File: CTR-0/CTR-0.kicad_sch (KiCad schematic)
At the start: 34 parts, among them J1 USB_C_Receptacle_USB2.0_14P, J2 Conn_01x20, J3 Conn_01x20, J4 Conn_01x03, SW1 SW_Push, U1 RP2040, U2 NCP1117-3.3_SOT223, U3 W25Q128JVS, Y1 12MHz

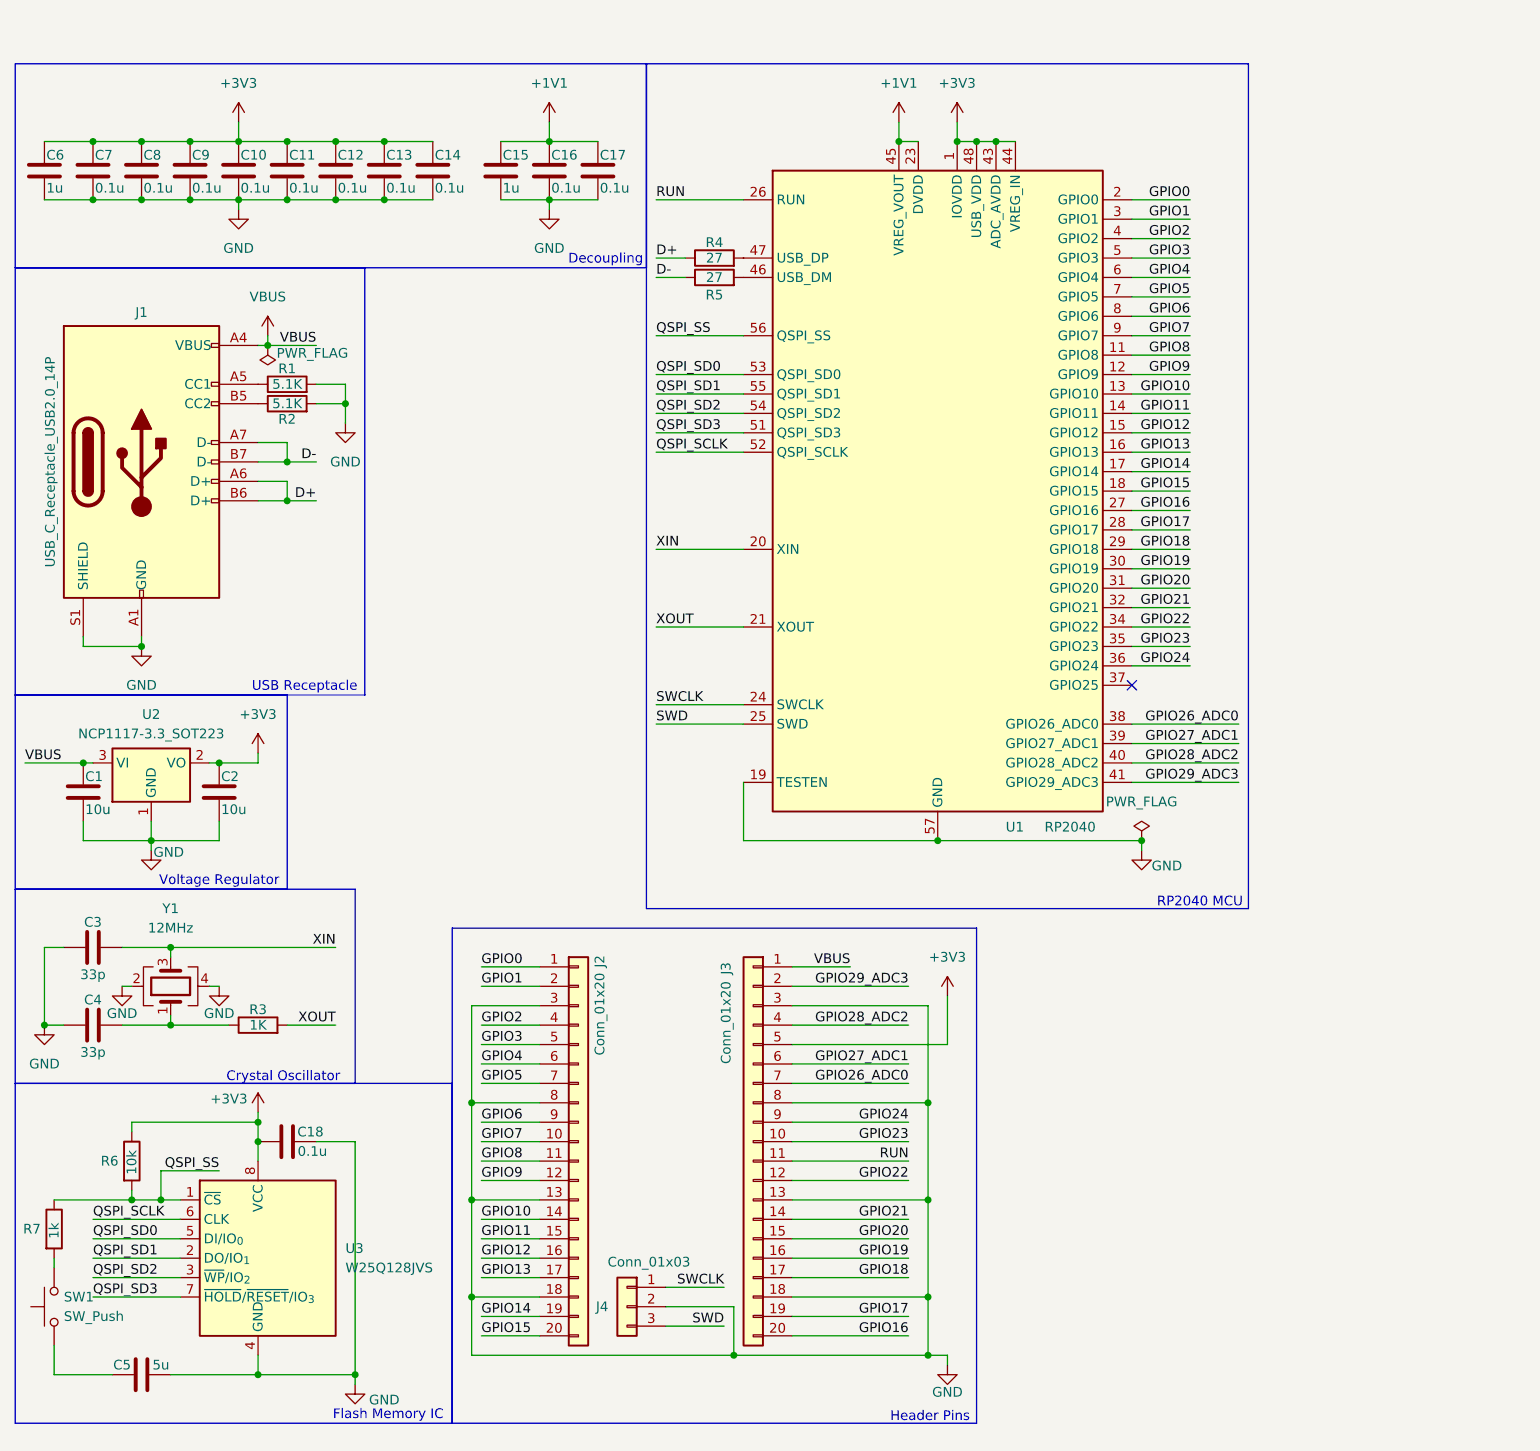
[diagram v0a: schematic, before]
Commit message: fixed push
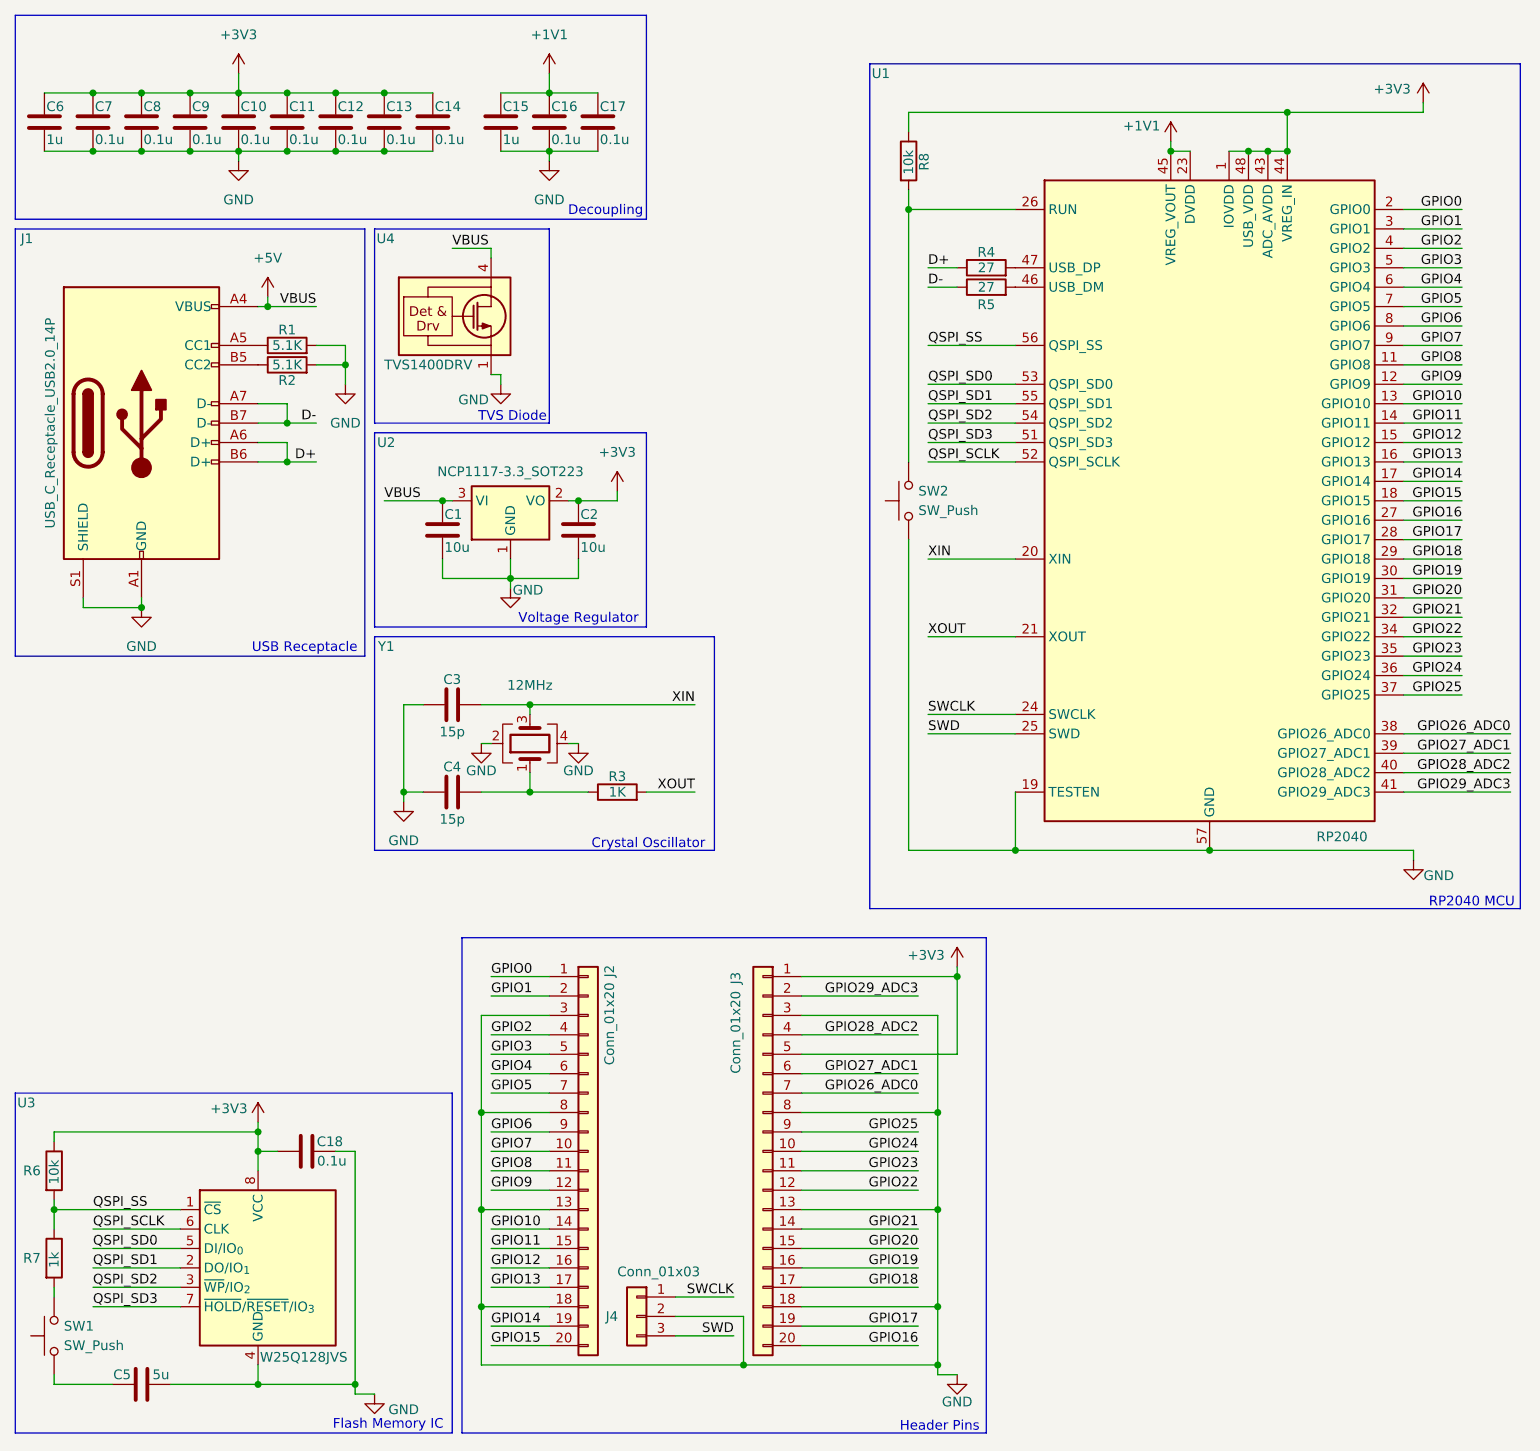
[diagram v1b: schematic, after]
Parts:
- added R8: 10k, Resistor_SMD:R_0402_1005Metric, symbol Device:R
- added SW2: SW_Push, Button_Switch_SMD:SW_Push_SPST_NO_Alps_SKRK, symbol Switch:SW_Push
- added U4: TVS1400DRV, Package_SON:WSON-6-1EP_2x2mm_P0.65mm_EP1x1.6mm, symbol Power_Protection:TVS1400DRV
- C3, C4: value 33p -> 15p
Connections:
- net +3V3: now also J3.1 (Pin_1), R8.1
- net GND: now also SW2.1, U4.1 (GND), U4.2 (GND), U4.3 (GND), U4.7 (GND)
- net GPIO23: now also J3.11 (Pin_11); no longer J3.10 (Pin_10)
- net GPIO24: now also J3.10 (Pin_10); no longer J3.9 (Pin_9)
- net GPIO25: now reaches U1.37 (GPIO25)
- net GPIO25: now also J3.9 (Pin_9)
- net RUN: no longer names the net of U1.26 (RUN)
- net RUN: now also R8.2, SW2.2; no longer J3.11 (Pin_11)
- net VBUS renamed +5V
- net +5V: now also U4.4 (IN), U4.5 (IN), U4.6 (IN); no longer J3.1 (Pin_1)
- no-connect marks 1 -> 0
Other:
- note added: "TVS Diode"
- moved on the sheet: C1, C10, C11, C12, C13, C14, C15, C16, C17, C18, C2, C3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

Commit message: Add files via upload
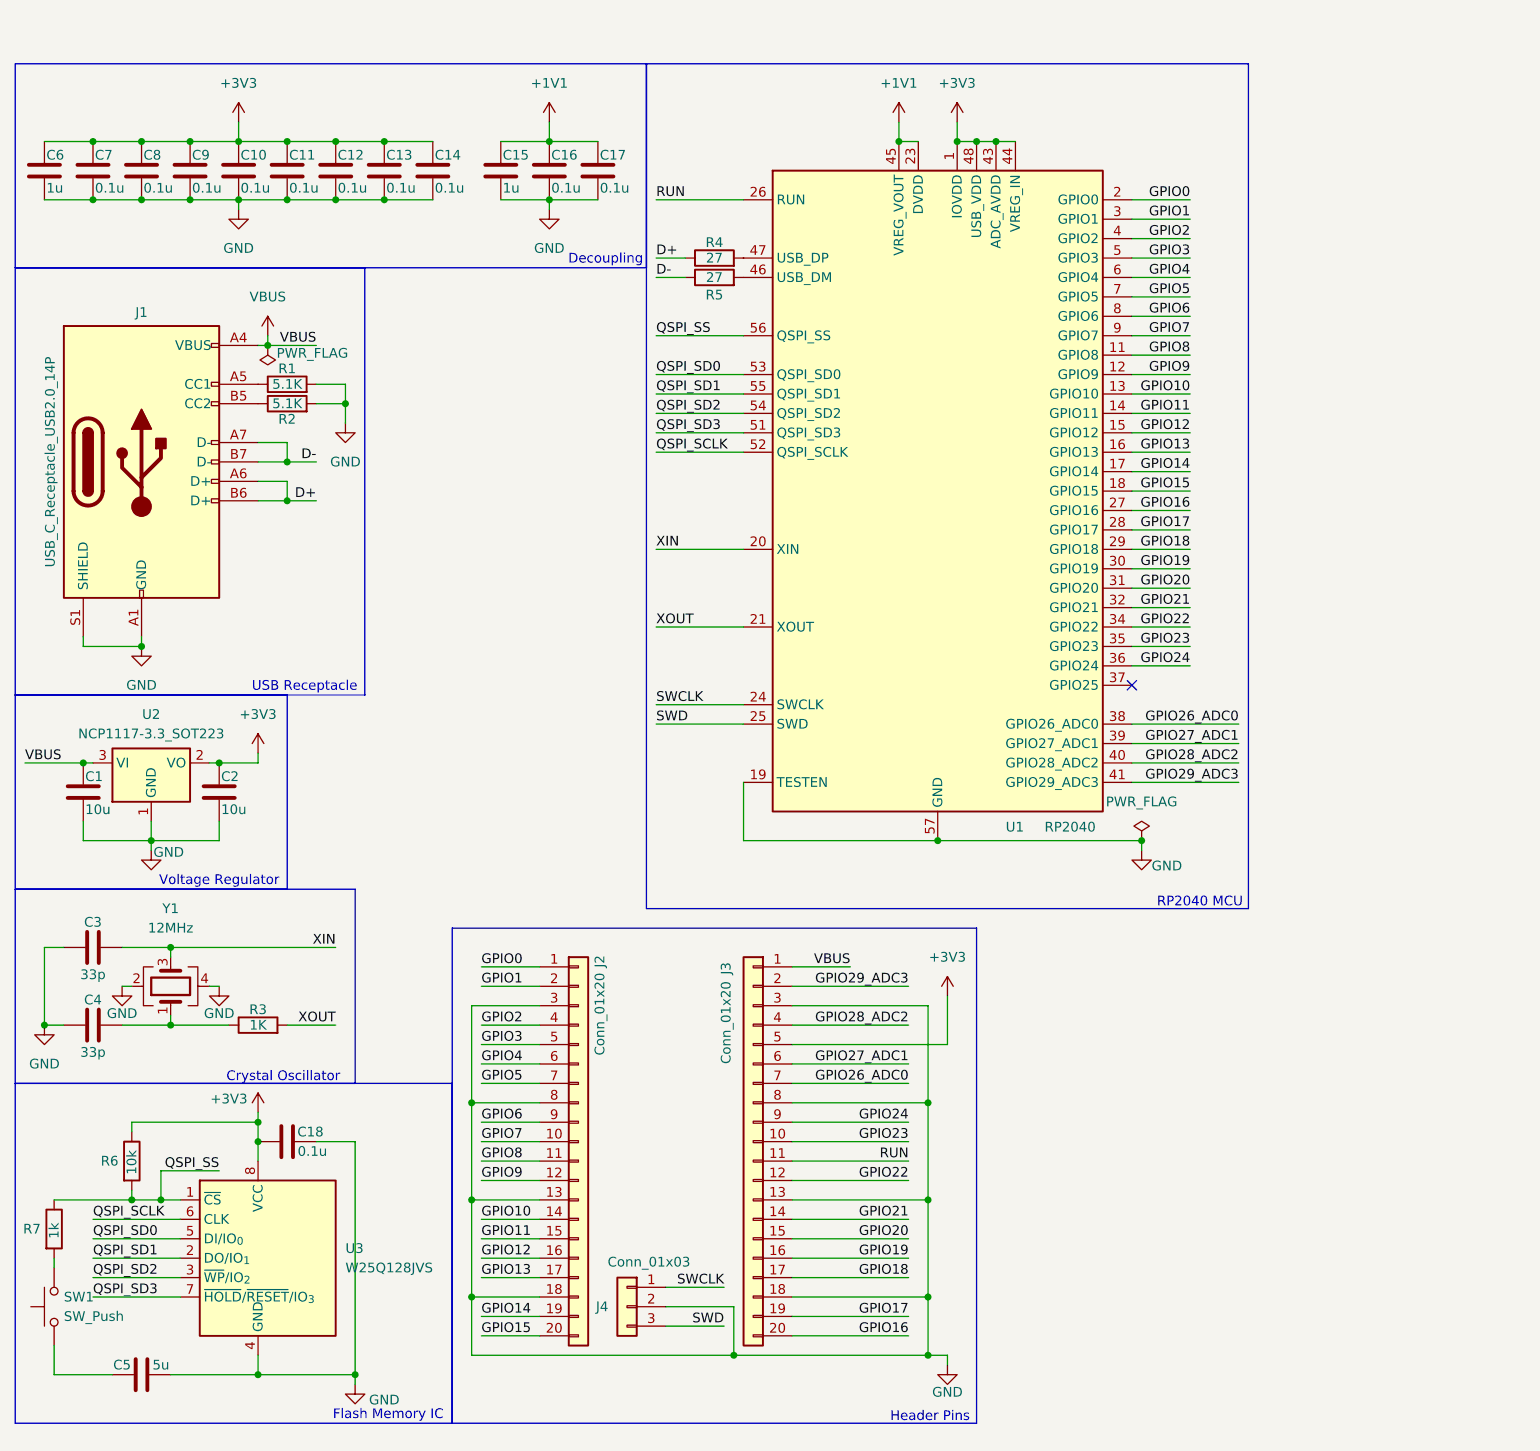
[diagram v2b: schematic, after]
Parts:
- removed R8: 10k, Resistor_SMD:R_0402_1005Metric, symbol Device:R
- removed SW2: SW_Push, Button_Switch_SMD:SW_Push_SPST_NO_Alps_SKRK, symbol Switch:SW_Push
- removed U4: TVS1400DRV, Package_SON:WSON-6-1EP_2x2mm_P0.65mm_EP1x1.6mm, symbol Power_Protection:TVS1400DRV
- C3, C4: value 15p -> 33p
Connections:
- net +3V3: no longer J3.1 (Pin_1)
- net GPIO23: now also J3.10 (Pin_10); no longer J3.11 (Pin_11)
- net GPIO24: now also J3.9 (Pin_9); no longer J3.10 (Pin_10)
- net RUN: now reaches U1.26 (RUN)
- net RUN: now also J3.11 (Pin_11)
- net +5V renamed VBUS
- net VBUS: now also J3.1 (Pin_1)
- net GPIO25: no longer names the net of U1.37 (GPIO25)
- net GPIO25: no longer J3.9 (Pin_9)
- no-connect marks 0 -> 1
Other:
- note removed: "TVS Diode"
- moved on the sheet: C1, C10, C11, C12, C13, C14, C15, C16, C17, C18, C2, C3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
